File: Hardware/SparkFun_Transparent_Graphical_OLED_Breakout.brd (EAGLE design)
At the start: 25.4 x 25.4 mm, 66 parts, among them U1 AP3012, U2 UG-2856KLBAG01_4WSPI

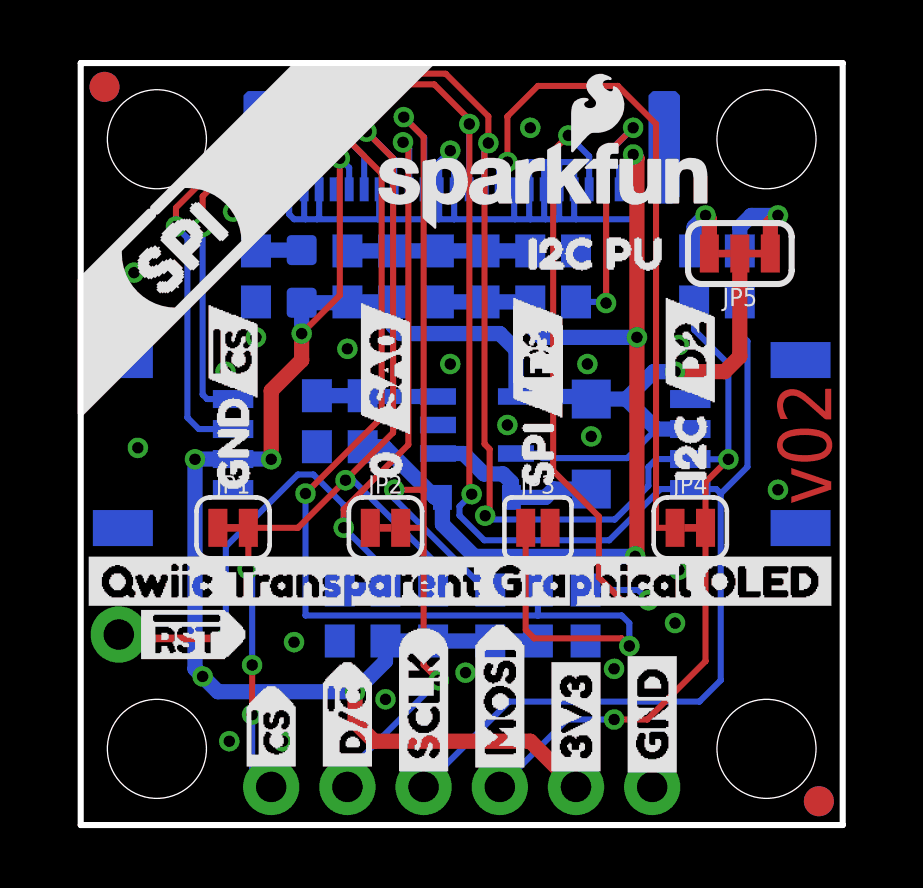
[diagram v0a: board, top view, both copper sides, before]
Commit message: Tidy schematic
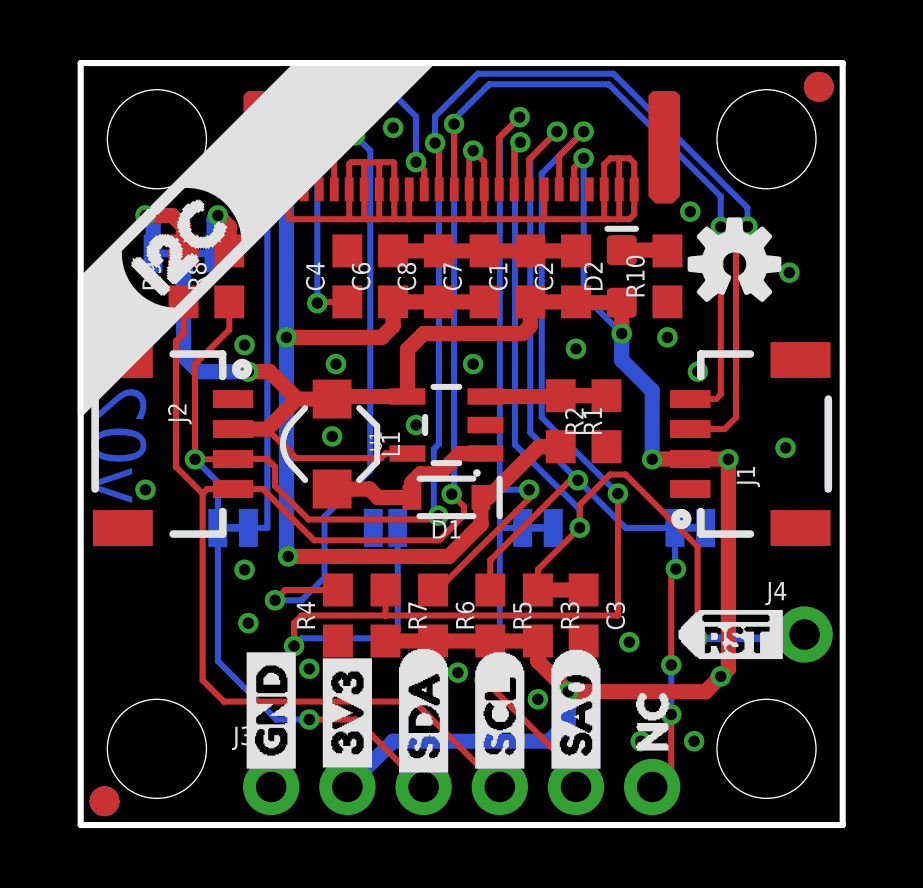
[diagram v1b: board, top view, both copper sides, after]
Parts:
- moved FRAME1 48.3 mm to (-11.4, -10.2), flipped to the top
- moved U$2 25.9 mm to (25.7, 8.13), flipped to the bottom
- moved FD1 23.8 mm to (0.79, 0.79), flipped to the top
- moved FD2 23.8 mm to (0.79, 0.79), flipped to the bottom
- moved FD3 23.8 mm to (24.6, 24.6), flipped to the top
- moved FD4 23.8 mm to (24.6, 24.6), flipped to the bottom
- moved U$19 23.1 mm to (1.14, 17.1), flipped to the top
- moved J4 22.9 mm to (24.1, 6.35), flipped to the top
- moved U$24 22.9 mm to (24.1, 17.1), flipped to the bottom
- moved U$17 22.7 mm to (24.0, 6.35), flipped to the bottom
- moved JP5 18.5 mm to (3.43, 19.1), flipped to the bottom
- moved R9 18.5 mm to (3.43, 18.3), flipped to the top
- moved LOGO2 18.2 mm to (21.8, 18.7), flipped to the top
- moved R8 15.5 mm to (4.95, 18.3), flipped to the top
- moved J1 15.2 mm to (20.3, 12.7), flipped to the top
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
